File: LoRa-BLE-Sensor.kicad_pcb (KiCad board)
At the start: 4 copper layers, 91 x 60 mm, 129 parts, among them J1 SHF-105-01-X-D-SM, J10 Battery_with_NTC, J11 Conn_01x02_Socket, J12 Conn_01x02_Socket, J2 Conn_01x02_Socket, J3 Battery_with_NTC, J4 Conn_01x06_Socket, J5 Screw_Terminal_01x06, J6 Screw_Terminal_01x06, J7 Screw_Terminal_01x04, J8 Conn_01x04_Pin, J9 Conn_01x04_Pin, Q1 DMN67D7L, Q10 SQ2389ES, Q11 SQ2389ES, Q12 DMN62D0UDW-7, Q13 DMN62D0UDW-7, Q2 DMN67D7L, Q3 DMN67D7L, Q4 DMN67D7L, Q5 DMN67D7L, Q6 DMN67D7L, Q7 DMN67D7L, Q8 DMN67D7L, Q9 SQ2389ES, SW1 SW_Push, SW2 SW_Push, SW3 SW_Push, U1 RAK4630, U2 NPM1300-QEAA-R, U3 TLV61046ADBVR, U4 TLV61046ADBVR, U5 TLV61046ADBVR

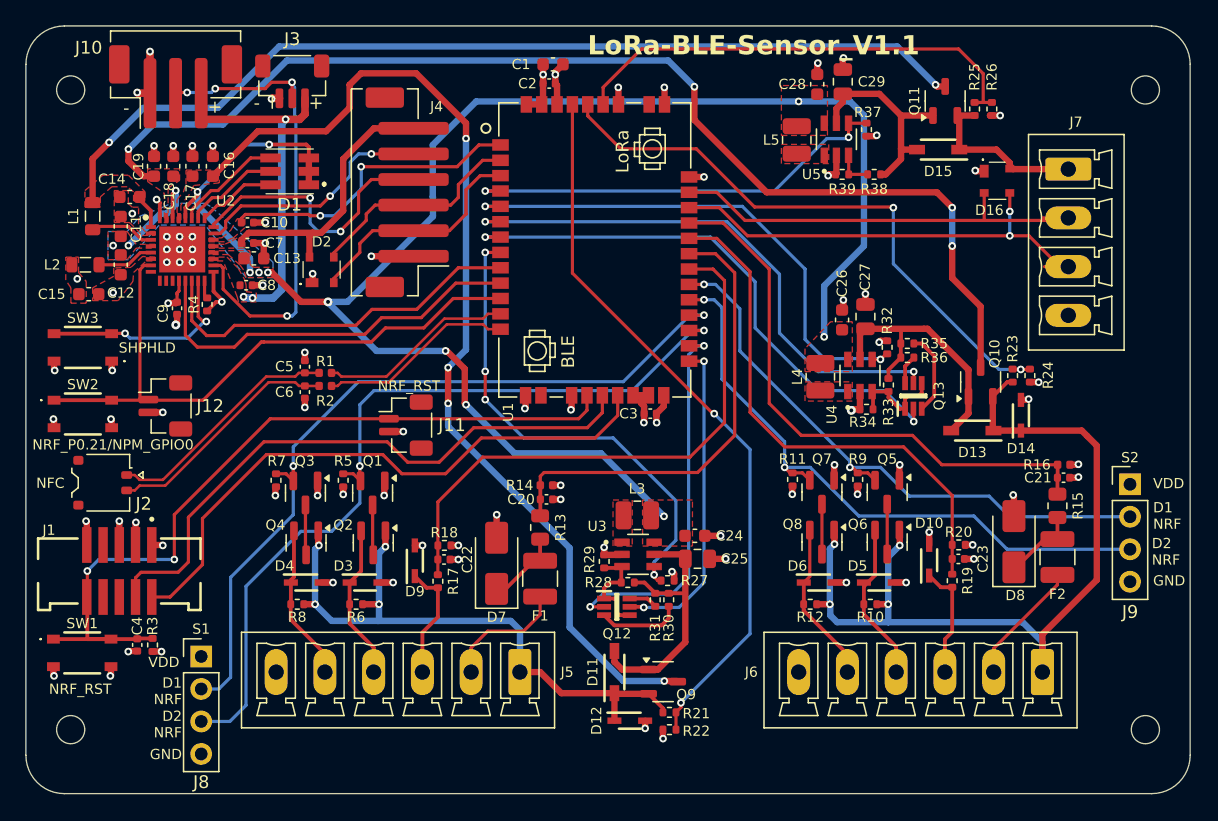
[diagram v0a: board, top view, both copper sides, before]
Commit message: added docs and manufacturing V1.1
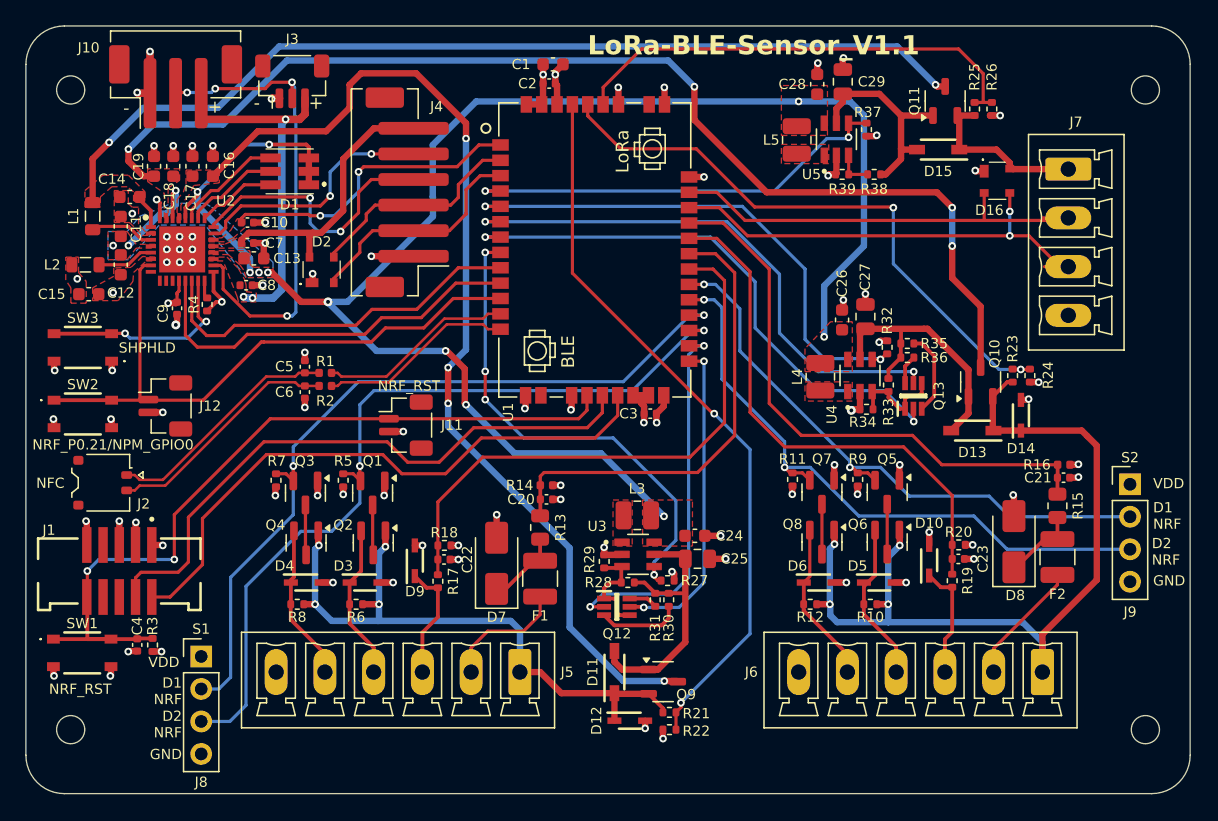
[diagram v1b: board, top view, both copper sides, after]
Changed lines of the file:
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@@
 	(paper "A4")
 	(title_block
-		(title "LoRa-BLE-Sensor")
-		(date "2025-03-05")
+		(title "LoRa-BLE-Sensor V1.1")
+		(date "2025-05-28")
 		(rev "1")
-		(company "Cyber Jungle")
+		(company "TerraMatrix")
 	)
 	(layers
@@
 			(drillshape 0)
 			(scaleselection 1)
-			(outputdirectory "Manufacturing/LoRa-BLE-Sensor_V1.0_Gerber/")
+			(outputdirectory "Manufacturing/LoRa-BLE-Sensor_V1.1/LoRa-BLE-Sensor_V1.1_Gerber/")
 		)
 	)
@@
 			(effects
 				(font
-					(size 1 1)
+					(size 0.8 0.8)
 					(thickness 0.15)
 				)
@@
 			(effects
 				(font
-					(size 1 1)
+					(size 0.8 0.8)
 					(thickness 0.15)
 				)
@@
 			(effects
 				(font
-					(size 1 1)
+					(size 0.8 0.8)
 					(thickness 0.15)
 				)
@@
 			(effects
 				(font
-					(size 1 1)
+					(size 0.8 0.8)
 					(thickness 0.15)
 				)
@@
 			(effects
 				(font
-					(size 1 1)
+					(size 0.8 0.8)
 					(thickness 0.15)
 				)
@@
 			(effects
 				(font
-					(size 1 1)
+					(size 0.8 0.8)
 					(thickness 0.15)
 				)
@@
 			(effects
 				(font
-					(size 1 1)
+					(size 0.8 0.8)
 					(thickness 0.15)
 				)
@@
 			(effects
 				(font
-					(size 1 1)
+					(size 0.8 0.8)
 					(thickness 0.15)
 				)
@@
 			(effects
 				(font
-					(size 1 1)
+					(size 0.8 0.8)
 					(thickness 0.15)
 				)
@@
 			(effects
 				(font
-					(size 1 1)
+					(size 0.8 0.8)
 					(thickness 0.15)
 				)
@@
 			(effects
 				(font
-					(size 1 1)
+					(size 0.8 0.8)
 					(thickness 0.15)
 				)
@@
 			(effects
 				(font
-					(size 1 1)
+					(size 0.8 0.8)
 					(thickness 0.15)
 				)
@@
 			(effects
 				(font
-					(size 1 1)
+					(size 0.8 0.8)
 					(thickness 0.15)
 				)
@@
 			(effects
 				(font
-					(size 1 1)
+					(size 0.8 0.8)
 					(thickness 0.15)
 				)
@@
 			(effects
 				(font
-					(size 1 1)
+					(size 0.8 0.8)
 					(thickness 0.15)
 				)
@@
 			(effects
 				(font
-					(size 1 1)
+					(size 0.8 0.8)
 					(thickness 0.15)
 				)
@@
 			(effects
 				(font
-					(size 1 1)
+					(size 0.8 0.8)
 					(thickness 0.15)
 				)
@@
 			(effects
 				(font
-					(size 1 1)
+					(size 0.8 0.8)
 					(thickness 0.15)
 				)
@@
 			(effects
 				(font
-					(size 1 1)
+					(size 0.8 0.8)
 					(thickness 0.15)
 				)
@@
 			(effects
 				(font
-					(size 1.27 1.27)
-					(thickness 0.254)
+					(size 0.8 0.8)
+					(thickness 0.15)
 				)
 			)
@@
 			(effects
 				(font
-					(size 1 1)
+					(size 0.8 0.8)
 					(thickness 0.15)
 				)
@@
 			(effects
 				(font
-					(size 1 1)
+					(size 0.8 0.8)
 					(thickness 0.15)
 				)
@@
 			(effects
 				(font
-					(size 1 1)
+					(size 0.8 0.8)
 					(thickness 0.15)
 				)
@@
 			(effects
 				(font
-					(size 1 1)
+					(size 0.8 0.8)
 					(thickness 0.15)
 				)
@@
 		)
 	)
-	(gr_text_box "Vo2"
+	(gr_text_box "Vo3"
 		(start 149.835 57.48)
 		(end 152.25375 62.09)
@@
 	(segment
 		(start 87.7825 62.2975)
-		(end 89.35 60.73)
+		(end 87.7825 60.4175)
 		(width 0.25)
 		(layer "B.Cu")
@@
 	)
 	(segment
-		(start 89.35 60.73)
-		(end 89.35 59.65)
+		(start 87.7825 60.4175)
+		(end 89.2 59)
 		(width 0.25)
 		(layer "B.Cu")
@@
 	)
 	(segment
-		(start 89.35 59.65)
-		(end 90 59)
-		(width 0.25)
-		(layer "B.Cu")
-		(net 14)
-	)
-	(segment
-		(start 90 59)
+		(start 89.2 59)
 		(end 91 59)
 		(width 0.25)
@@
 	)
 	(segment
-		(start 99.4 58.3)
-		(end 101.094853 58.3)
+		(start 97.7 60)
+		(end 99.4 58.3)
 		(width 0.25)
 		(layer "F.Cu")
@@
 	)
 	(segment
-		(start 97.7 60)
-		(end 99.4 58.3)
+		(start 87.015 63.834669)
+		(end 86.215 63.834669)
+		(width 0.25)
+		(layer "F.Cu")
+		(net 17)
+	)
+	(segment
+		(start 90 60.4)
+		(end 90.4 60)
 		(width 0.25)
 		(layer "F.Cu")
@@
 	)
 	(segment
-		(start 90.2 60)
+		(start 90.4 60)
 		(end 97.7 60)
 		(width 0.25)
@@
 	)
 	(segment
-		(start 87.015 63.834669)
-		(end 86.215 63.834669)
+		(start 99.4 58.3)
+		(end 101.094853 58.3)
 		(width 0.25)
 		(layer "F.Cu")
@@
 	)
 	(via
-		(at 90.2 60)
+		(at 90 60.4)
 		(size 0.6)
 		(drill 0.3)
@@
 	)
 	(segment
-		(start 87.015 63.834669)
-		(end 88.110331 63.834669)
-		(width 0.25)
-		(layer "B.Cu")
-		(net 17)
-	)
-	(segment
-		(start 90.215 61.73)
-		(end 90.215 60.015)
+		(start 88.110331 63.834669)
+		(end 87.015 63.834669)
 		(width 0.25)
 		(layer "B.Cu")
@@
 	)
 	(segment
-		(start 88.110331 63.834669)
-		(end 90.215 61.73)
+		(start 90 60.4)
+		(end 90 61.945)
 		(width 0.25)
 		(layer "B.Cu")
@@
 	)
 	(segment
-		(start 90.215 60.015)
-		(end 90.2 60)
+		(start 90 61.945)
+		(end 88.110331 63.834669)
 		(width 0.25)
 		(layer "B.Cu")
